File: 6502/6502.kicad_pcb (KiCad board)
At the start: 2 copper layers, 158.8 x 185.4 mm, 51 parts, among them J1 Conn_01x08, J10 Conn_02x20_Odd_Even, J11 Jack-DC, J12 Conn_01x02, J2 Conn_01x08, J3 Conn_01x03, J4 Conn_02x20_Odd_Even, J5 Conn_01x08, J6 Conn_01x03, J7 Conn_02x20_Odd_Even, J8 Conn_02x20_Odd_Even, J9 Mini-DIN-6, Q1 FQP47P06, SW1 SW_Push, SW2 SW_Push, U1 74LS08, U2 74LS154, U3 28C256, U4 ATF22V10C, U5 65C02S, U6 AS6C4008-55PCN, U7 6522, U8 6522, U9 NHD-0420H1Z, X1 ACO-4MHz

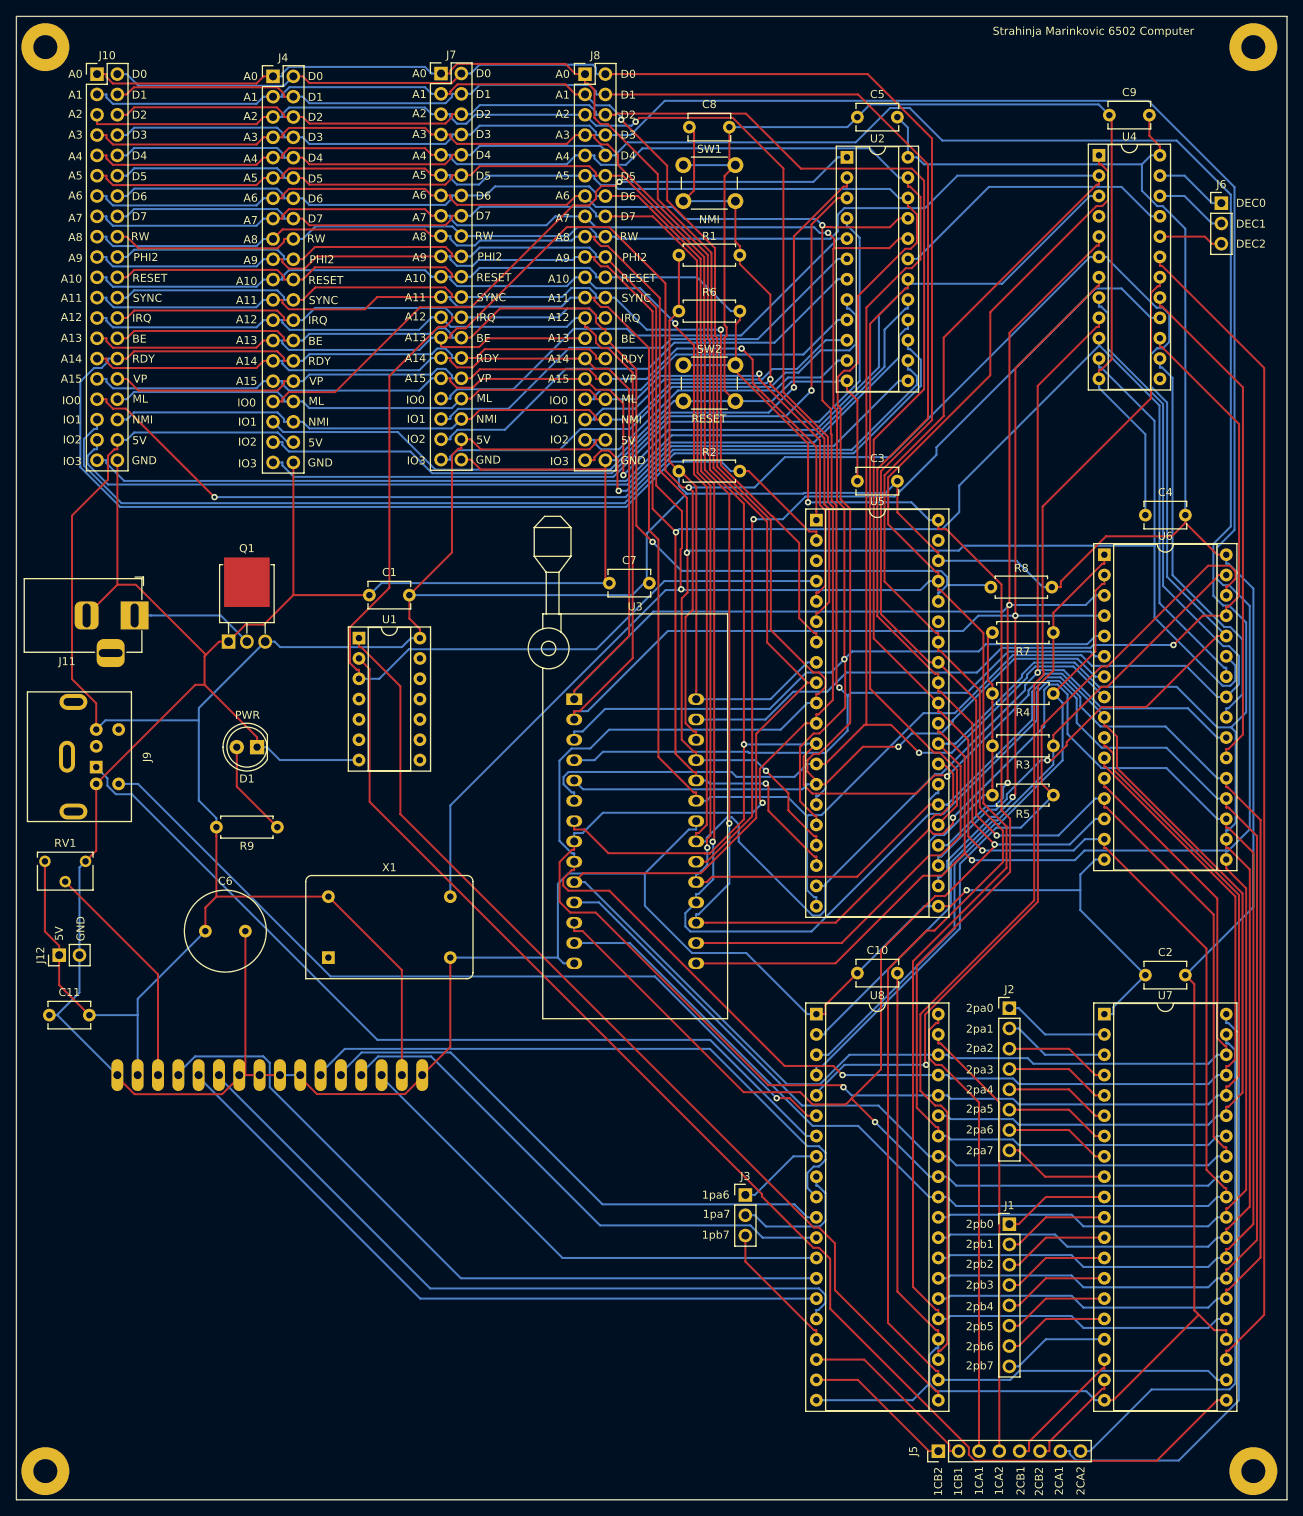
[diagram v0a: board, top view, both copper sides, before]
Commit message: changes
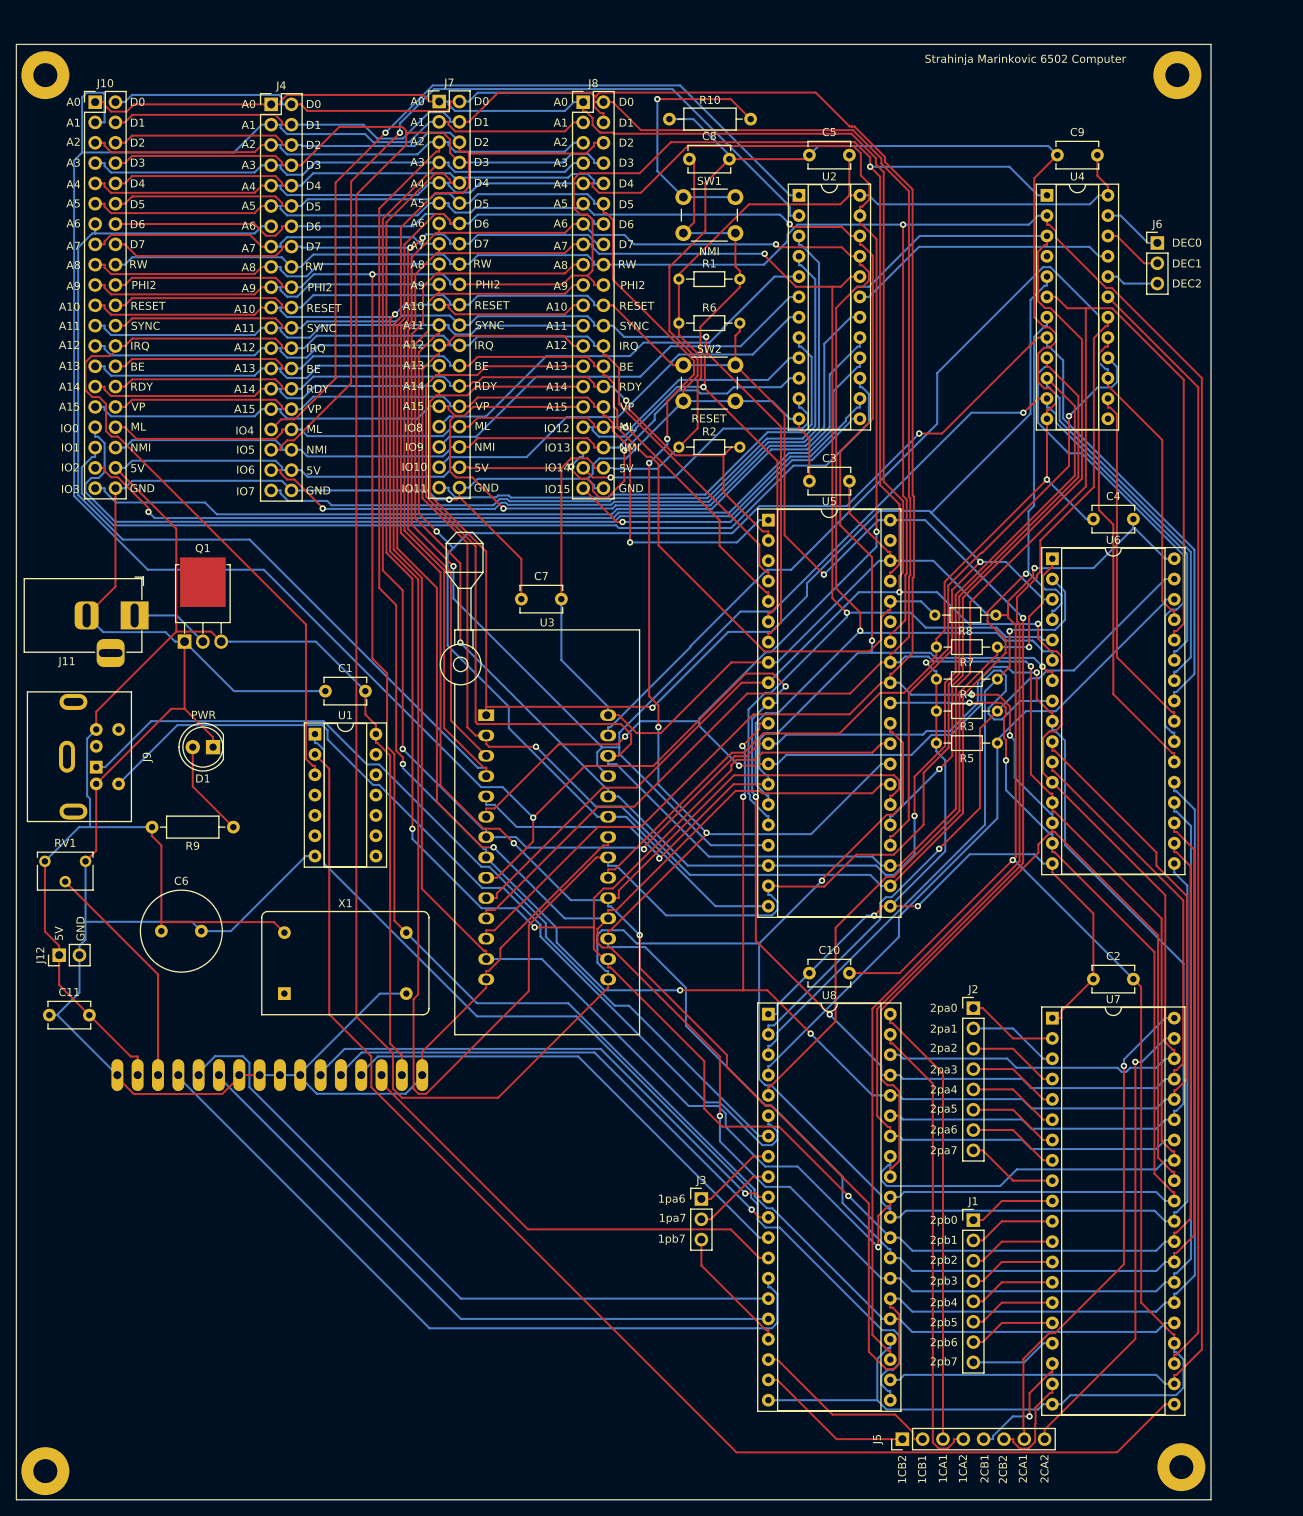
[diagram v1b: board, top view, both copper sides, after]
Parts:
- added R10: 220Ω, Resistor_THT:R_Axial_DIN0207_L6.3mm_D2.5mm_P10.16mm_Horizontal, F.Cu at (210.0, 90.0)
- R1, R2, R3, R4, R5, R6, R7, R8: footprint Resistor_THT:R_Axial_DIN0207_L6.3mm_D2.5mm_P7.62mm_Horizontal -> Resistor_THT:R_Axial_DIN0204_L3.6mm_D1.6mm_P7.62mm_Horizontal
- R9: footprint Resistor_THT:R_Axial_DIN0207_L6.3mm_D2.5mm_P7.62mm_Horizontal -> Resistor_THT:R_Axial_DIN0207_L6.3mm_D2.5mm_P10.16mm_Horizontal
- moved C1 13.2 mm to (167.0, 161.5)
- moved U1 13.2 mm to (165.7, 166.9)
- moved C7 11.2 mm to (191.5, 150.0)
- moved U3 11.2 mm to (187.1, 164.5)
- moved REF2 10.1 mm to (273.5, 84.5)
- moved R5 9.55 mm to (251.0, 168.0)
- moved J6 9.42 mm to (271.0, 105.5)
- moved REF3 9.01 mm to (274.0, 258.5)
- moved R3 8.24 mm to (251.0, 164.0)
- moved C9 8.20 mm to (258.5, 94.5)
- moved U4 8.20 mm to (257.2, 99.5)
- moved R8 7.83 mm to (243.2, 152.0)
- moved C5 7.65 mm to (227.5, 94.5)
- moved U2 7.65 mm to (226.2, 99.5)
- moved R7 7.23 mm to (251.0, 156.0)
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- renumbered REF** to REF1, REF** to REF2, REF** to REF3, REF** to REF4
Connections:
- SW1 pad 1: GND -> Net-(SW1-Pad1)
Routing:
- net a6: track 248.7 -> 359.5 mm
- net a10: track 286.5 -> 383.6 mm, vias 2 -> 1
- net RDY: track 182.4 -> 99.5 mm, vias 0 -> 1
- net +5V: track 782.8 -> 706.6 mm, vias 0 -> 2
- net d7: track 348.3 -> 397.3 mm, vias 1 -> 4
- net a1: track 348.1 -> 392.5 mm, vias 2 -> 4
- net d4: track 420.5 -> 379.1 mm, vias 0 -> 3
- net Net-(SW1-Pad1): track 0.00 -> 32.8 mm, vias 0 -> 1
- net GND: track 682.8 -> 652.0 mm, vias 1 -> 5
- net d1: track 354.1 -> 380.8 mm
- net a9: track 272.7 -> 298.6 mm
- net a15: track 234.4 -> 258.5 mm, vias 1 -> 2
- net WE: track 111.4 -> 134.9 mm, vias 1 -> 0
- net RW: track 345.5 -> 368.7 mm, vias 0 -> 1
- net ML: track 117.2 -> 96.7 mm
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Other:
- board size 158.8 x 185.4 mm -> 149.3 x 181.9 mm
